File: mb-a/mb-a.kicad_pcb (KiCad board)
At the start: 2 copper layers, 39 x 56 mm, 29 parts, among them J1 Power, J2 Speaker, M1 Orange-Pi-Zero, U1 NCP1117-5.0_SOT223, U2 PAM8320, X1 I2C-6P

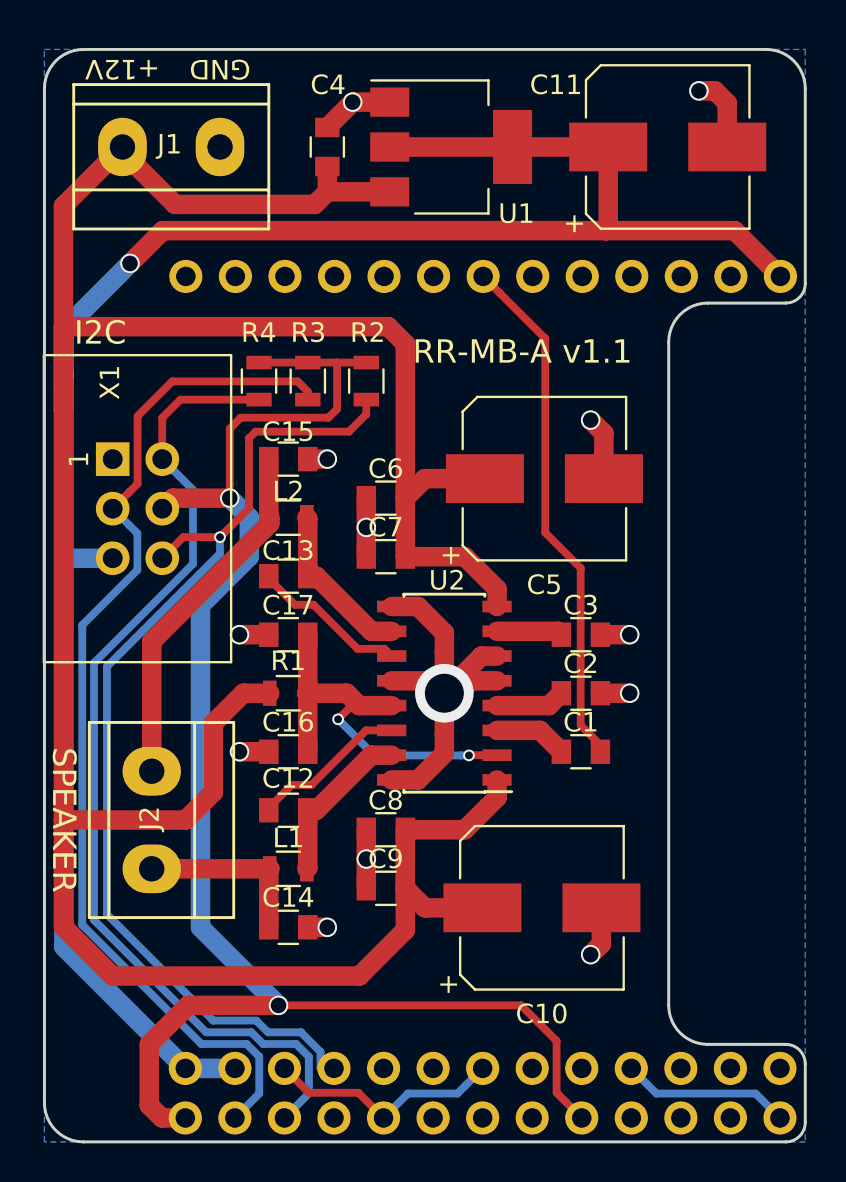
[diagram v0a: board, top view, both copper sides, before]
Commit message: WIP
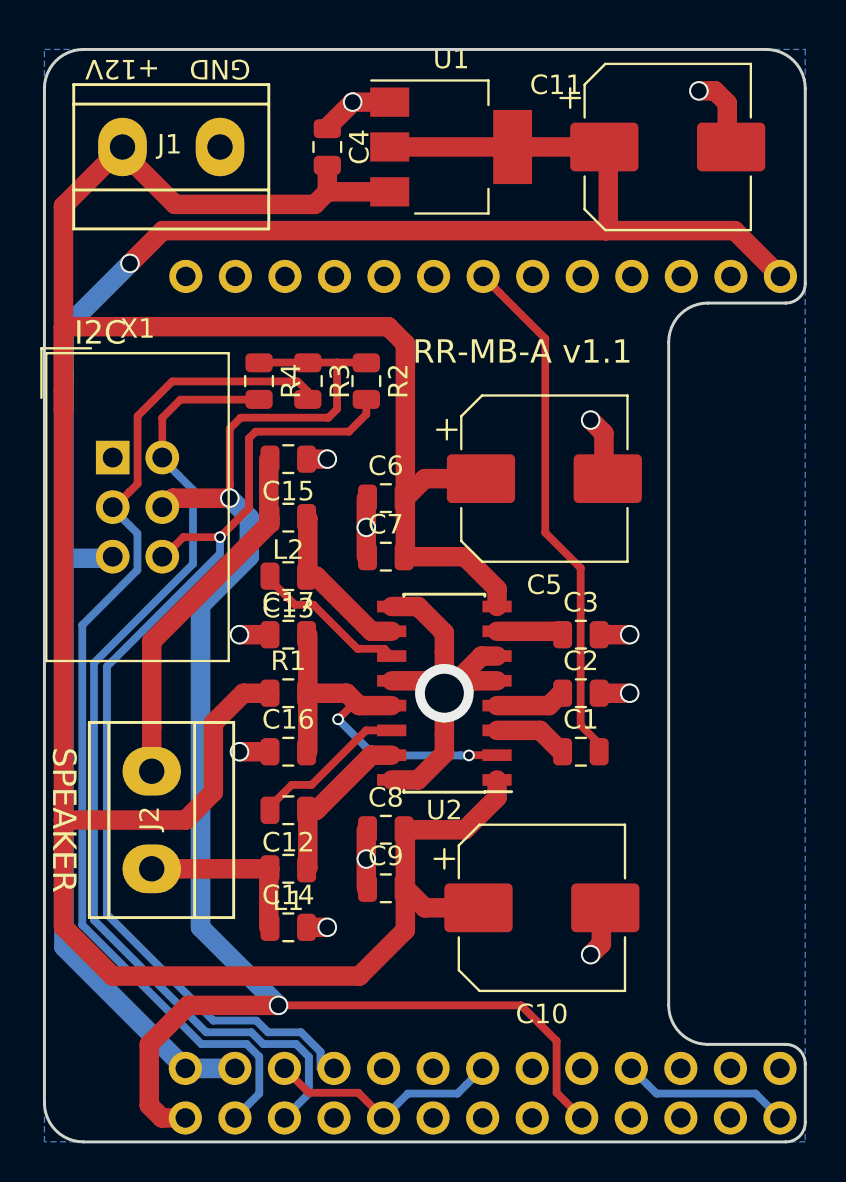
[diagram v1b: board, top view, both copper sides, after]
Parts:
- C1, C12, C13, C14, C15, C16, C17, C2, C3, C4, C6, C7, C8, C9: footprint Capacitors_SMD:C_0805 -> Capacitor_SMD:C_0805_2012Metric
- C10, C11, C5: footprint Capacitors_SMD:CP_Elec_8x10 -> Capacitor_SMD:CP_Elec_8x10
- L1, L2: footprint Inductors_SMD:L_0805 -> Inductor_SMD:L_0805_2012Metric
- R1, R2, R3, R4: footprint Resistors_SMD:R_0805 -> Resistor_SMD:R_0805_2012Metric
- U1: footprint TO_SOT_Packages_SMD:SOT-223-3Lead_TabPin2 -> Package_TO_SOT_SMD:SOT-223-3_TabPin2
- U2: footprint Housings_SOIC:SOIC-16_3.9x9.9mm_Pitch1.27mm -> Package_SO:SOIC-16_3.9x9.9mm_P1.27mm
- X1: footprint Connectors:IDC_Header_Straight_6pins -> Connector_IDC:IDC-Header_2x03_P2.54mm_Vertical
- moved X1 0.08 mm to (95.0, 60.9), turned to 0 degrees
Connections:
- M1 pad 10: (no net) -> Net-(M1-Pad10)
- M1 pad 11: (no net) -> Net-(M1-Pad11)
- M1 pad 12: (no net) -> Net-(M1-Pad12)
- M1 pad 13: (no net) -> Net-(M1-Pad13)
- M1 pad 15: (no net) -> Net-(M1-Pad15)
- M1 pad 16: (no net) -> Net-(M1-Pad16)
- M1 pad 18: (no net) -> Net-(M1-Pad18)
- M1 pad 19: (no net) -> Net-(M1-Pad19)
- M1 pad 21: (no net) -> Net-(M1-Pad21)
- M1 pad 22: (no net) -> Net-(M1-Pad22)
- M1 pad 23: (no net) -> Net-(M1-Pad23)
- M1 pad 24: (no net) -> Net-(M1-Pad24)
- M1 pad 26: (no net) -> Net-(M1-Pad26)
- M1 pad 29: (no net) -> Net-(M1-Pad29)
- M1 pad 30: (no net) -> Net-(M1-Pad30)
- M1 pad 31: (no net) -> Net-(M1-Pad31)
- M1 pad 32: (no net) -> Net-(M1-Pad32)
- M1 pad 34: (no net) -> Net-(M1-Pad34)
- M1 pad 35: (no net) -> Net-(M1-Pad35)
- M1 pad 36: (no net) -> Net-(M1-Pad36)
- M1 pad 37: (no net) -> Net-(M1-Pad37)
- M1 pad 38: (no net) -> Net-(M1-Pad38)
- M1 pad 39: (no net) -> Net-(M1-Pad39)
- M1 pad 7: (no net) -> Net-(M1-Pad7)
